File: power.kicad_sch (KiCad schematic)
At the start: 37 parts, among them IC501 TPS51206DSQR, U501 TPS62130ARGTR, U502 TPS62130ARGTR, U503 SPX3819M5-L-3-3, U504 TPS62130ARGTR

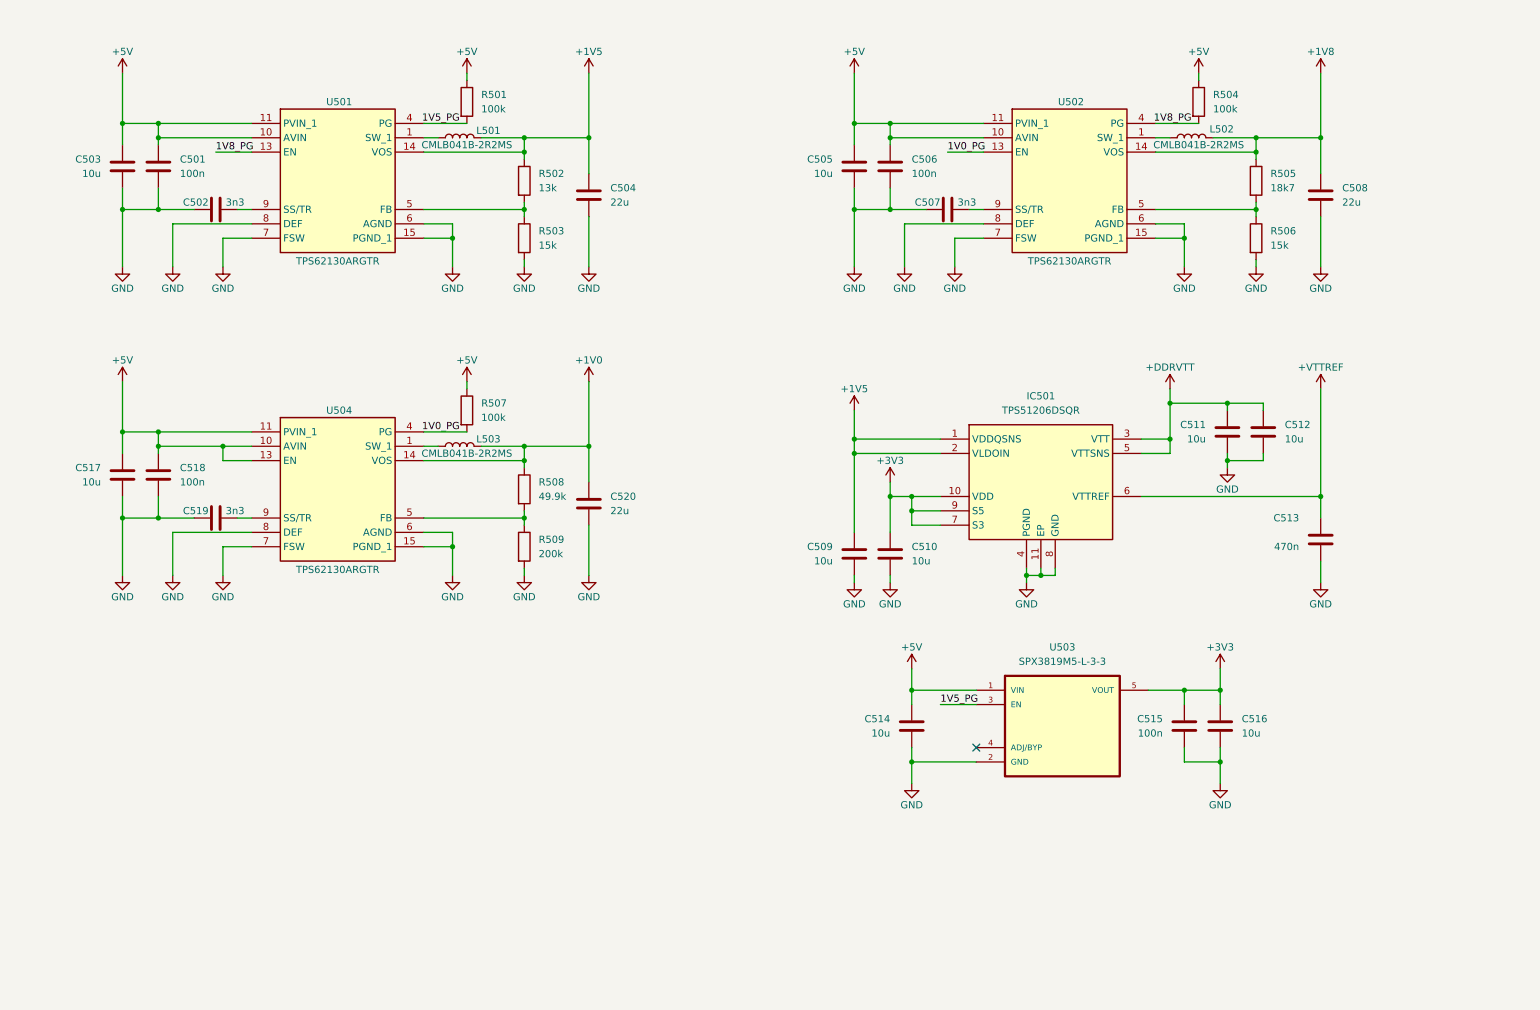
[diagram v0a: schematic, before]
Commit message: feat: continue ps mio sch design
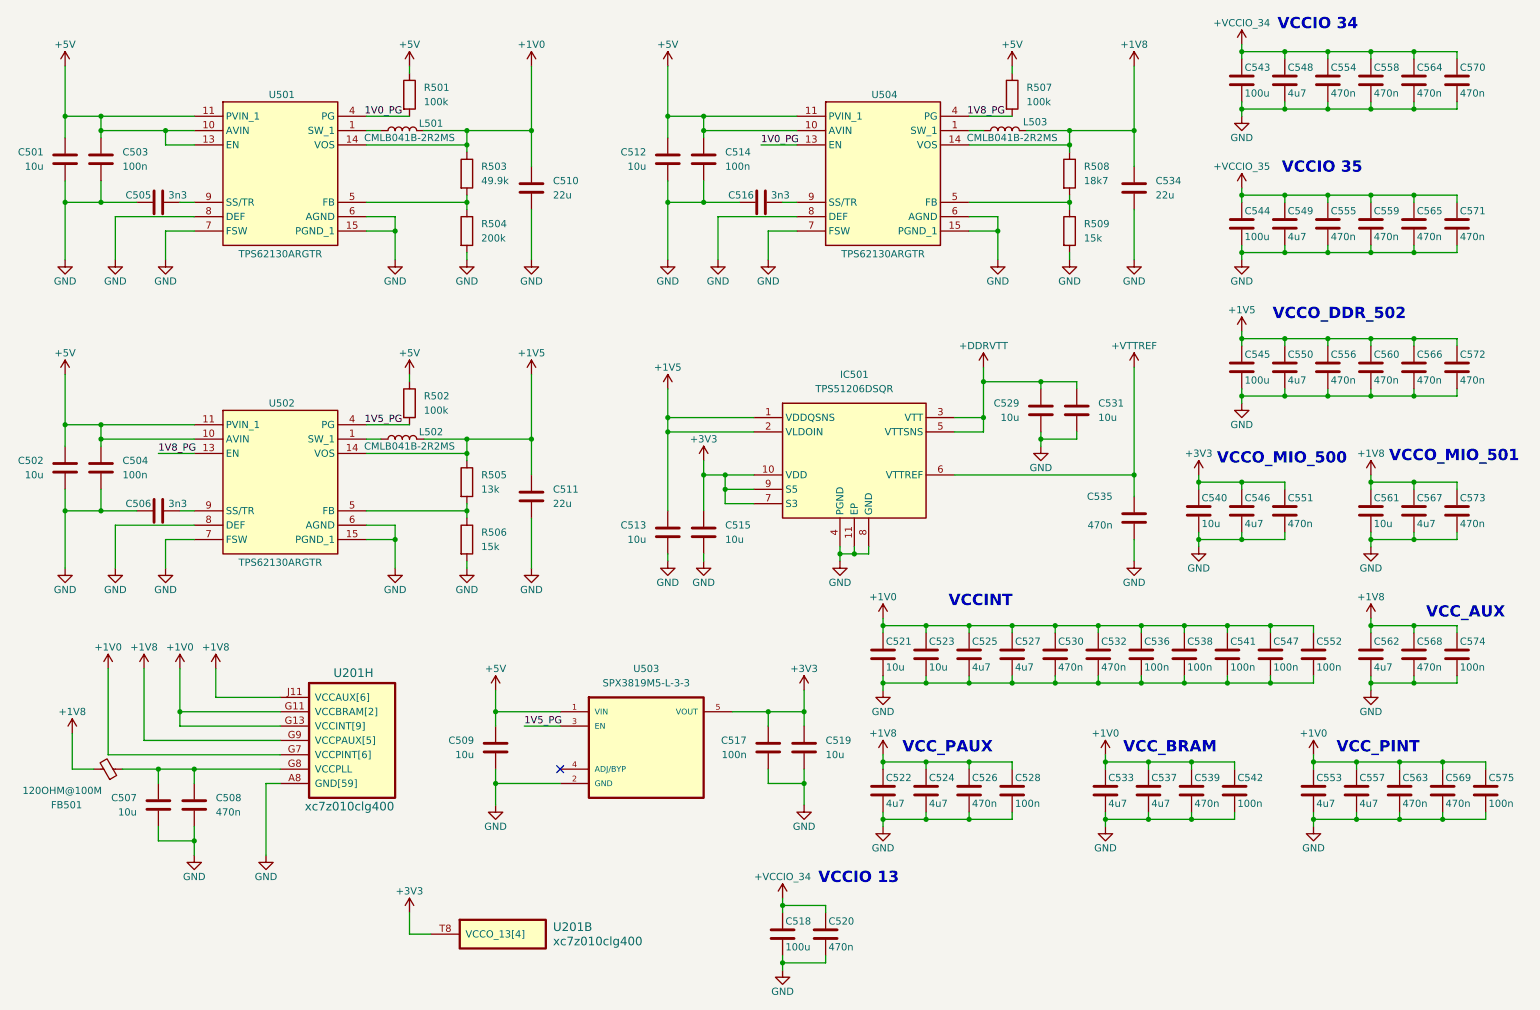
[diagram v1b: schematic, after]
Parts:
- added C507, C521, C523, C540, C561: 10u, Capacitor_SMD:C_0805_2012Metric, symbol Device:C
- added C508, C520, C526, C530, C532, C539, C551, C554, C555, C556, C558, C559, C560, C563, C564, C565, C566, C568, C569, C570, C571, C572, C573: 470n, Capacitor_SMD:C_0402_1005Metric, symbol Device:C
- added C518, C543, C544, C545: 100u, Capacitor_SMD:C_1206_3216Metric, symbol Device:C
- added C522, C524, C525, C527, C533, C537, C546, C548, C549, C550, C553, C557, C562, C567: 4u7, Capacitor_SMD:C_0603_1608Metric, symbol Device:C
- added C528, C536, C538, C541, C542, C547, C552, C574, C575: 100n, Capacitor_SMD:C_0402_1005Metric, symbol Device:C
- added FB501: 120OHM@100M, Inductor_SMD:L_0603_1608Metric, symbol Device:FerriteBead_Small
- added U201: xc7z010clg400, Package_BGA:Xilinx_CLG400, symbol Xilinx7:xc7z010clg400
- renumbered C517 to C501, C503 to C502, C518 to C503, C501 to C504, C519 to C505, C502 to C506, C514 to C509, C520 to C510, C504 to C511, C505 to C512, C509 to C513, C506 to C514, C510 to C515, C507 to C516, C515 to C517, C516 to C519, C511 to C529, C512 to C531, C508 to C534, C513 to C535, L503 to L501, L501 to L502, L502 to L503, R507 to R501, R501 to R502, R508 to R503, R509 to R504, R502 to R505, R503 to R506, R504 to R507, R505 to R508, R506 to R509, U504 to U501, U501 to U502, U502 to U504
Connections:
- net +1V0: now also C521.1, C523.1, C525.1, C527.1, C530.1, C532.1, C533.1, C536.1, C537.1, C538.1, C539.1, C541.1, C542.1, C547.1, C552.1, C553.1, C557.1, C563.1, C569.1, C575.1, U201.G11 (VCCBRAM[2]), U201.G13 (VCCINT[9]), U201.G7 (VCCPINT[6]), U201.H10 (VCCBRAM[2]), U201.H12 (VCCINT[9]), U201.J13 (VCCINT[9]), U201.J7 (VCCPINT[6]), U201.K12 (VCCINT[9]), U201.L13 (VCCINT[9]), U201.L7 (VCCPINT[6]), U201.M12 (VCCINT[9]), U201.N13 (VCCINT[9]), U201.N7 (VCCPINT[6]), U201.P12 (VCCINT[9]), U201.P8 (VCCPINT[6]), U201.R13 (VCCINT[9]), U201.R7 (VCCPINT[6])
- net +1V5: now also C545.1, C550.1, C556.1, C560.1, C566.1, C572.1
- net +1V8: now also C522.1, C524.1, C526.1, C528.1, C561.1, C562.1, C567.1, C568.1, C573.1, C574.1, FB501.2, U201.F8 (VCCPAUX[5]), U201.G9 (VCCPAUX[5]), U201.H8 (VCCPAUX[5]), U201.J11 (VCCAUX[6]), U201.K8 (VCCPAUX[5]), U201.L11 (VCCAUX[6]), U201.M8 (VCCPAUX[5]), U201.N11 (VCCAUX[6]), U201.N9 (VCCAUX[6]), U201.P10 (VCCAUX[6]), U201.R9 (VCCAUX[6])
- net +3V3: now also C540.1, C546.1, C551.1, U201.T8 (VCCO_13[4]), U201.U11 (VCCO_13[4]), U201.W7 (VCCO_13[4]), U201.Y10 (VCCO_13[4])
- net GND: now also C507.2, C508.2, C518.2, C520.2, C521.2, C522.2, C523.2, C524.2, C525.2, C526.2, C527.2, C528.2, C530.2, C532.2, C533.2, C536.2, C537.2, C538.2, C539.2, C540.2, C541.2, C542.2, C543.2, C544.2, C545.2, C546.2, C547.2, C548.2, C549.2, C550.2, C551.2, C552.2, C553.2, C554.2, C555.2, C556.2, C557.2, C558.2, C559.2, C560.2, C561.2, C562.2, C563.2, C564.2, C565.2, C566.2, C567.2, C568.2, C569.2, C570.2, C571.2, C572.2, C573.2, C574.2, C575.2, U201.A18 (GND[59]), U201.A8 (GND[59]), U201.B1 (GND[59]), U201.B11 (GND[59]), U201.C14 (GND[59]), U201.C4 (GND[59]), U201.C9 (GND[59]), U201.D17 (GND[59]), U201.E10 (GND[59]), U201.E20 (GND[59]), U201.F3 (GND[59]), U201.F7 (GND[59]), U201.G10 (GND[59]), U201.G12 (GND[59]), U201.G16 (GND[59]), U201.H11 (GND[59]), U201.H13 (GND[59]), U201.H19 (GND[59]), U201.H7 (GND[59]), U201.H9 (GND[59]), U201.J12 (GND[59]), U201.J2 (GND[59]), U201.J8 (GND[59]), U201.K11 (GND[59]), U201.K13 (GND[59]), U201.K15 (GND[59]), U201.K5 (GND[59]), U201.K7 (GND[59]), U201.L12 (GND[59]), U201.L18 (GND[59]), U201.L8 (GND[59]), U201.M1 (GND[59]), U201.M11 (GND[59]), U201.M13 (GND[59]), U201.M7 (GND[59]), U201.N10 (GND[59]), U201.N12 (GND[59]), U201.N14 (GND[59]), U201.N4 (GND[59]), U201.N8 (GND[59]), U201.P11 (GND[59]), U201.P13 (GND[59]), U201.P17 (GND[59]), U201.P7 (GND[59]), U201.P9 (GND[59]), U201.R12 (GND[59]), U201.R20 (GND[59]), U201.R8 (GND[59]), U201.T13 (GND[59]), U201.T3 (GND[59]), U201.T7 (GND[59]), U201.U16 (GND[59]), U201.U6 (GND[59]), U201.V19 (GND[59]), U201.V9 (GND[59]), U201.W12 (GND[59]), U201.W2 (GND[59]), U201.Y15 (GND[59]), U201.Y5 (GND[59])
- new net: C507.1, C508.1, FB501.1, U201.G8 (VCCPLL)
- new net +VCCIO_34: C518.1, C520.1, C543.1, C548.1, C554.1, C558.1, C564.1, C570.1
- new net +VCCIO_35: C544.1, C549.1, C555.1, C559.1, C565.1, C571.1
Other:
- note added: "VCCINT"
- note added: "VCCIO 13"
- note added: "VCCIO 34"
- note added: "VCCIO 35"
- note added: "VCCO_DDR_502"
- note added: "VCCO_MIO_500"
- note added: "VCCO_MIO_501"
- note added: "VCC_AUX"
- note added: "VCC_BRAM"
- note added: "VCC_PAUX"
- note added: "VCC_PINT"
- moved on the sheet: C501, C502, C503, C504, C505, C506, C509, C510, C511, C512, C513, C514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

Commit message: feat: continue improve sch design
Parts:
- FB501: footprint Inductor_SMD:L_0603_1608Metric -> Inductor_SMD:L_0402_1005Metric
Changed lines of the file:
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@@
 			)
 		)
-		(property "Footprint" "Inductor_SMD:L_0603_1608Metric"
+		(property "Footprint" "Inductor_SMD:L_0402_1005Metric"
 			(at 33.02 151.638 90)
 			(hide yes)
